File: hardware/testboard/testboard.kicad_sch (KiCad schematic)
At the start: 0 parts

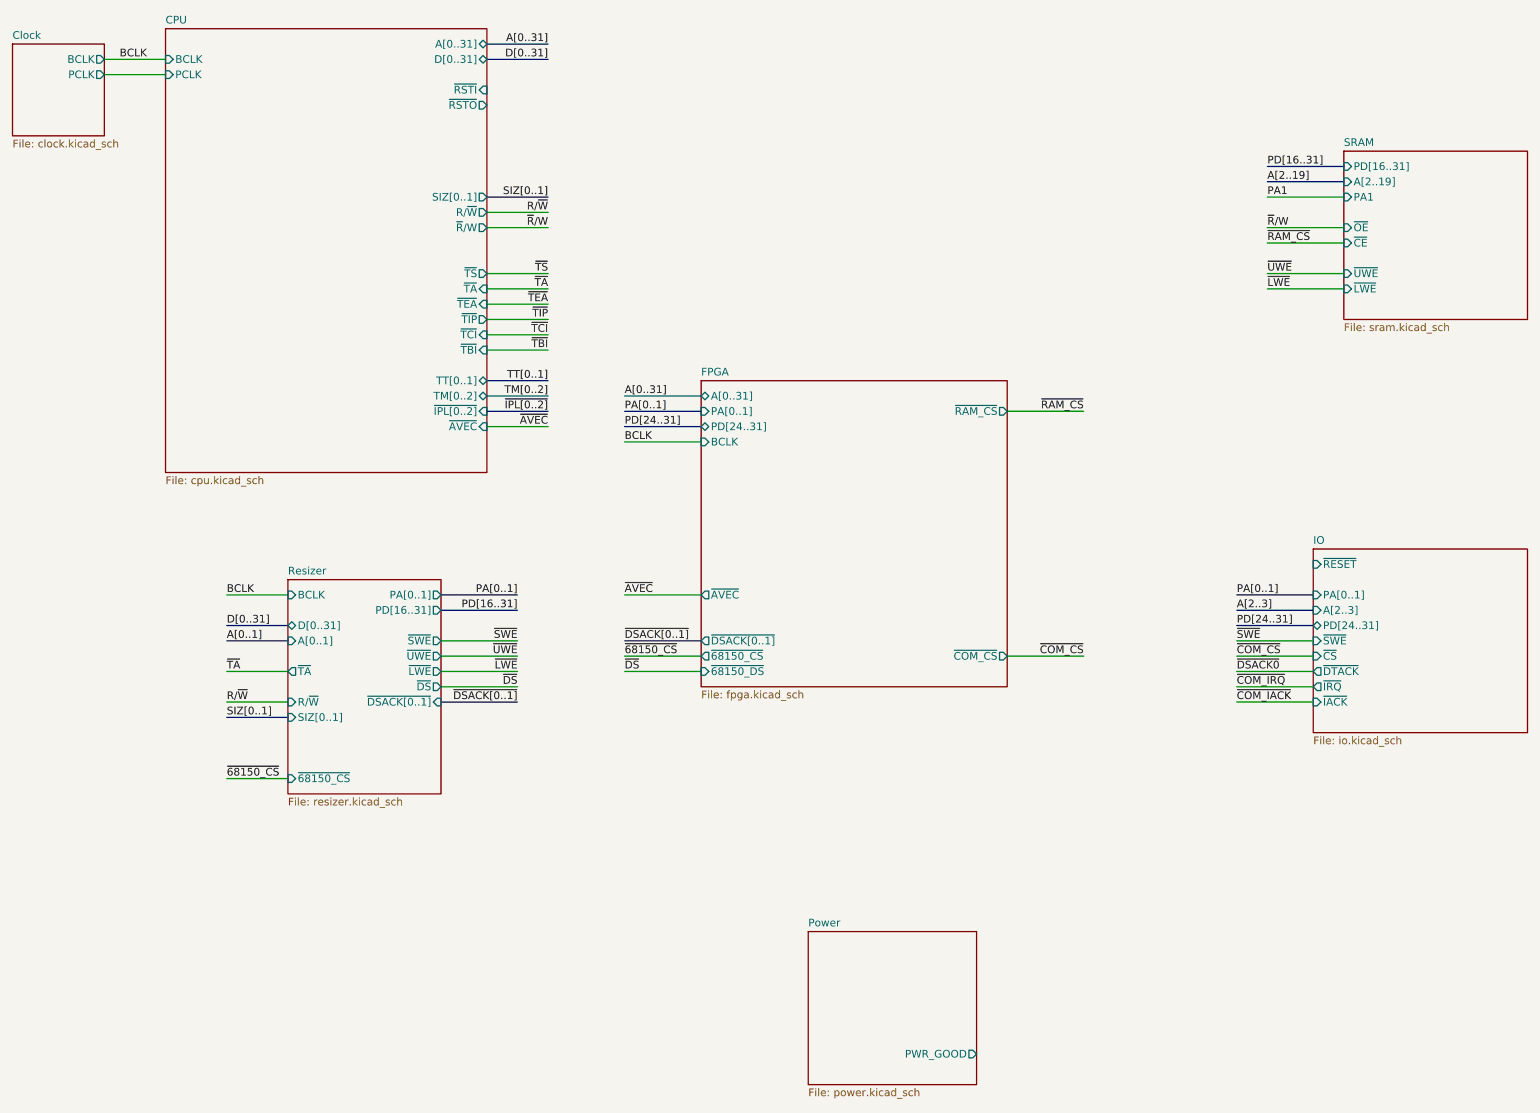
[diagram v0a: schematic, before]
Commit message: root mostly finished
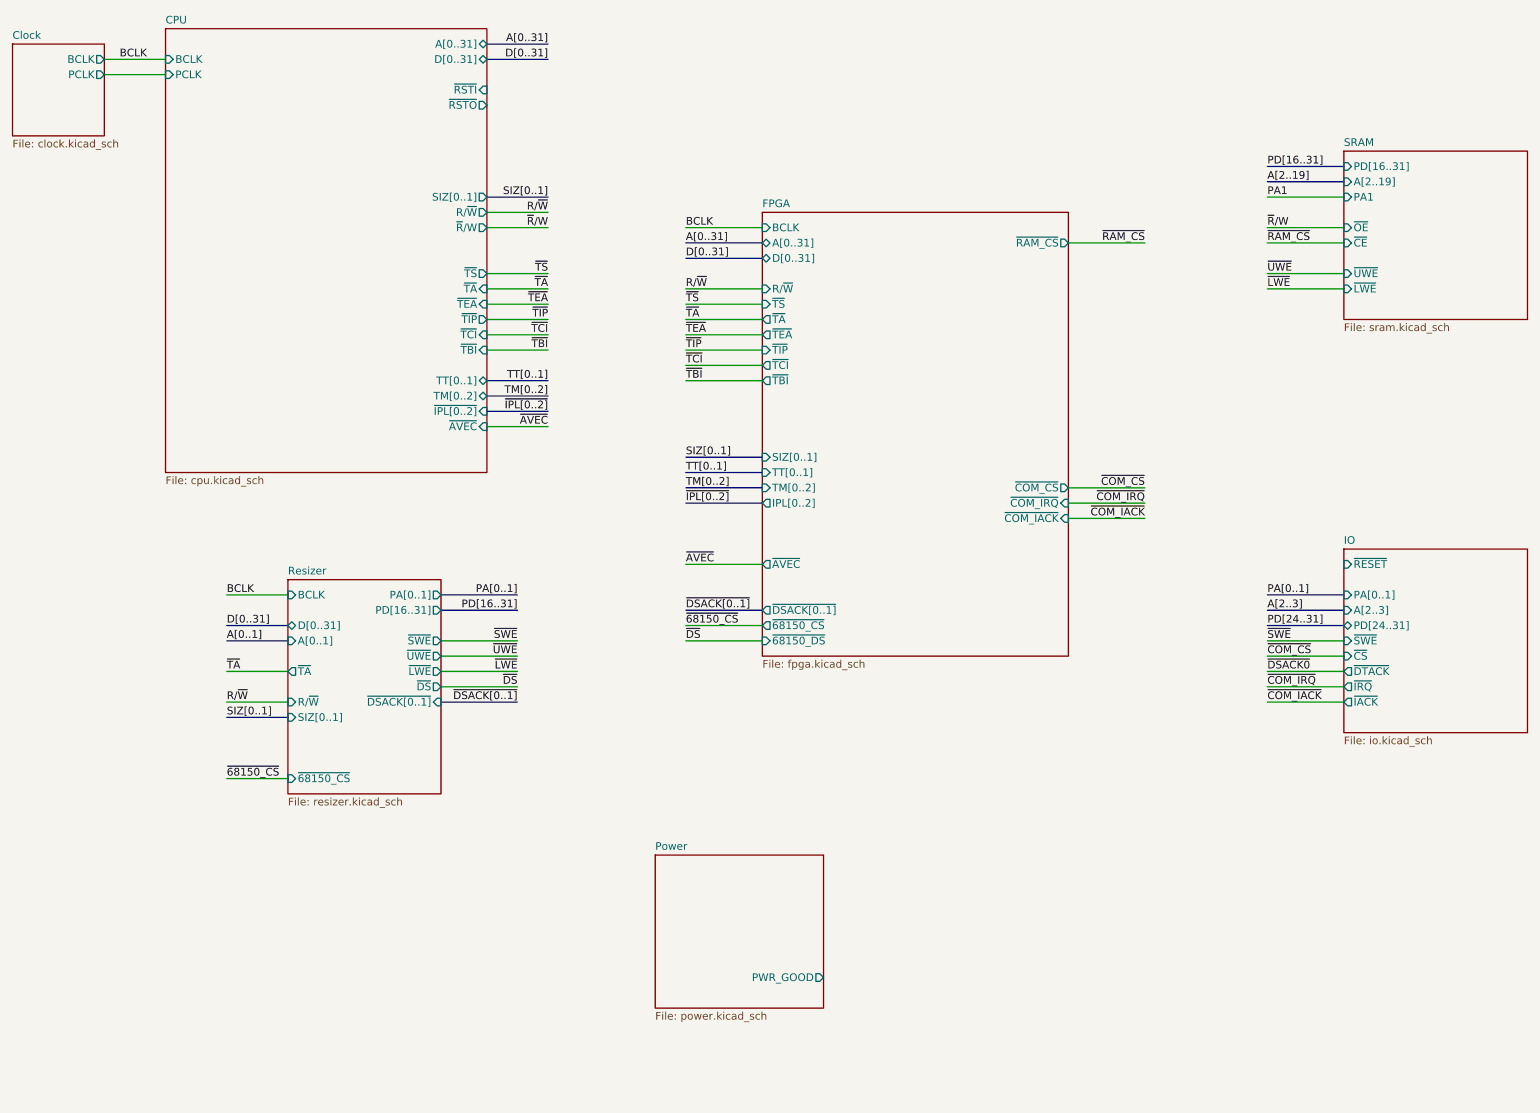
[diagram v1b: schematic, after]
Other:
- sheet FPGA ports: added D[0..31], IPL[0..2], R/~{W}, SIZ[0..1], TM[0..2], TT[0..1], ~{COM_IACK}, ~{COM_IRQ}, ~{TA}, ~{TBI}, ~{TCI}, ~{TEA}, ~{TIP}, ~{TS}; removed PA[0..1], PD[24..31]
